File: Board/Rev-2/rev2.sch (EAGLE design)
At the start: 52 parts, among them IC1 74HC595N, T1 2N3904, T2 2N3904, T3 2N3904, T4 2N3904, T5 2N3904, T6 2N3904, T7 2N3904, T8 2N3904

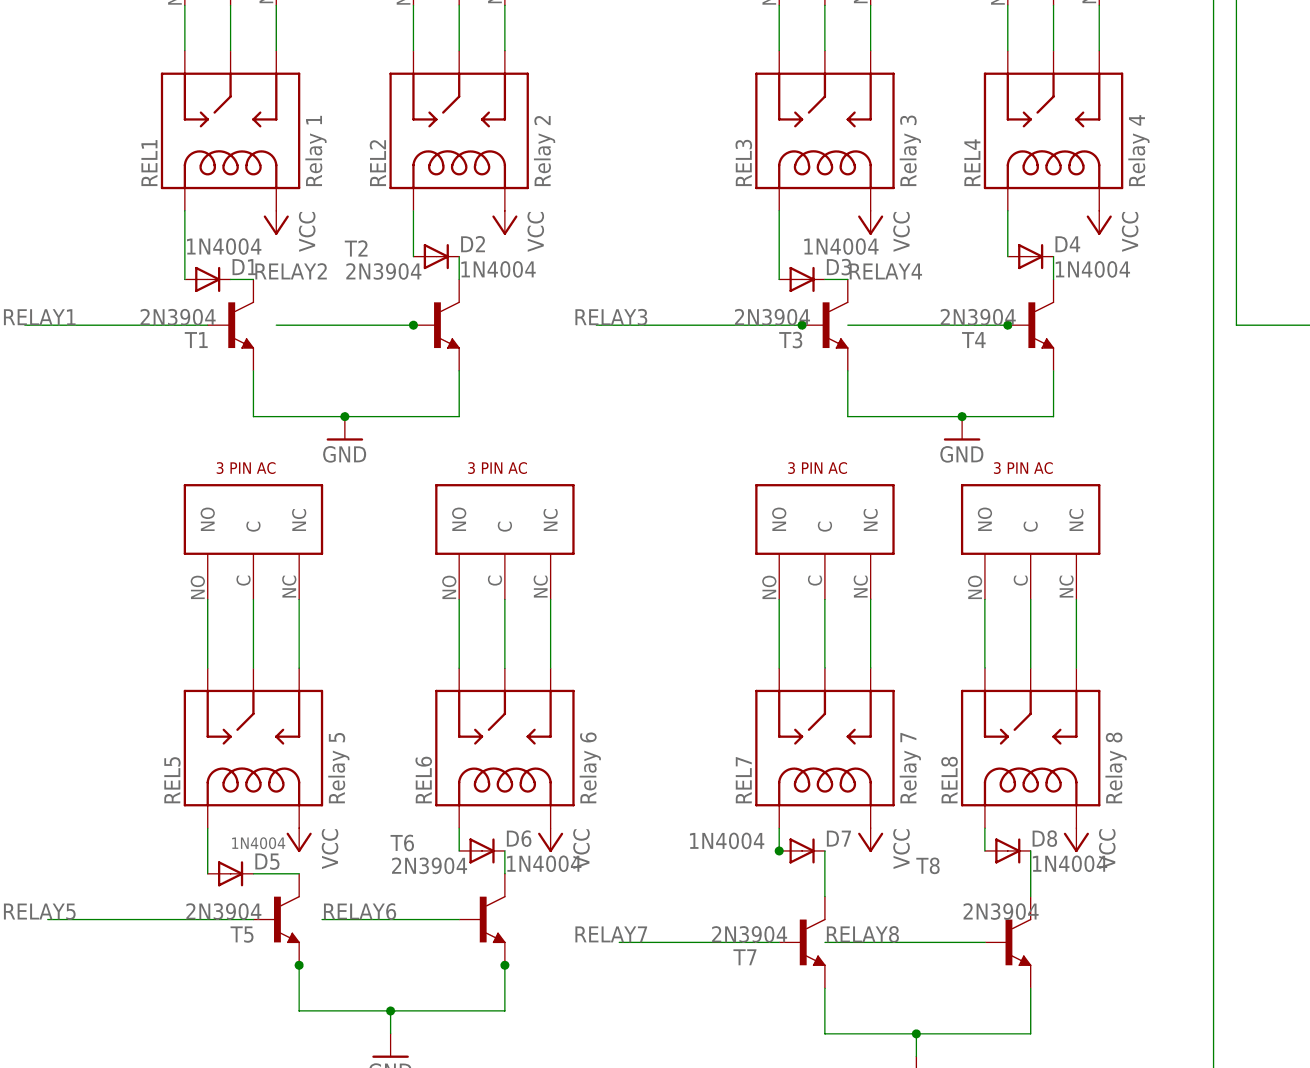
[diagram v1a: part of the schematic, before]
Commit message: Board Updates
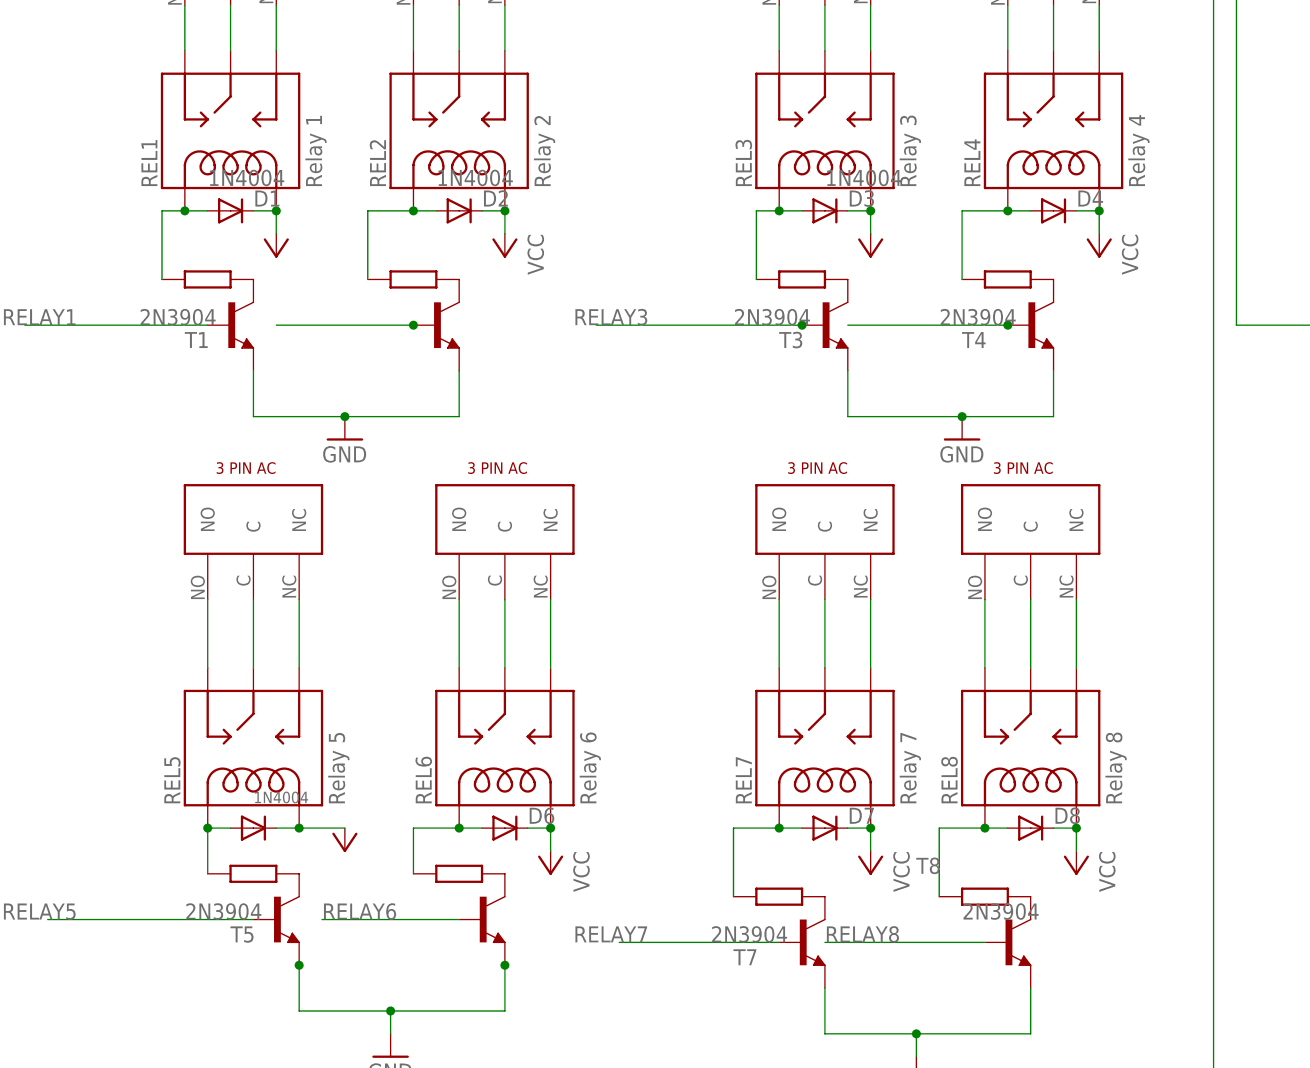
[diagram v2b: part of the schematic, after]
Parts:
- added LIMIT_REG_1, LIMIT_REG_2, LIMIT_REG_3, LIMIT_REG_4, LIMIT_REG_5, LIMIT_REG_6, LIMIT_REG_7, LIMIT_REG_8: 10 ohm, resistor:R-EU_0204/7
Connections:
- removed net N$47: D1.C, T1.C
- removed net N$48: D2.C, T2.C
- removed net N$49: D3.C, T3.C
- removed net N$50: D4.C, T4.C
- removed net N$51: D8.C, T8.C
- removed net N$52: D7.C, T7.C
- removed net N$53: D6.C, T6.C
- removed net N$54: D5.A, REL5.COIL1
- new net N$30: LIMIT_REG_1.1, T1.C
- new net N$32: LIMIT_REG_3.1, T3.C
- new net N$33: LIMIT_REG_2.1, T2.C
- new net N$34: LIMIT_REG_4.1, T4.C
- new net N$35: LIMIT_REG_8.1, T8.C
- new net N$36: LIMIT_REG_7.1, T7.C
- new net N$37: LIMIT_REG_6.1, T6.C
- new net N$38: LIMIT_REG_5.1, T5.C
- net N$1: now also D5.A, LIMIT_REG_5.2, REL5.COIL1; no longer D1.A, REL1.COIL1
- net N$2: now also D6.A, LIMIT_REG_6.2, REL6.COIL1; no longer D2.A, REL2.COIL1
- net N$3: now also D7.A, LIMIT_REG_7.2, REL7.COIL1; no longer D3.A, REL3.COIL1
- net N$4: now also D8.A, LIMIT_REG_8.2, REL8.COIL1; no longer D4.A, REL4.COIL1
- net N$5: now also D4.A, LIMIT_REG_4.2, REL4.COIL1; no longer D5.C, T5.C
- net N$6: now also D3.A, LIMIT_REG_3.2, REL3.COIL1; no longer D6.A, REL6.COIL1
- net N$8: now also D2.A, LIMIT_REG_2.2, REL2.COIL1; no longer D7.A, REL7.COIL1
- net N$9: now also D1.A, LIMIT_REG_1.2, REL1.COIL1; no longer D8.A, REL8.COIL1
- net VCC: now also D1.C, D2.C, D3.C, D4.C, D5.C, D6.C, D7.C, D8.C
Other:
- moved on the sheet: D1, D2, D3, D4, D6, D7, D8

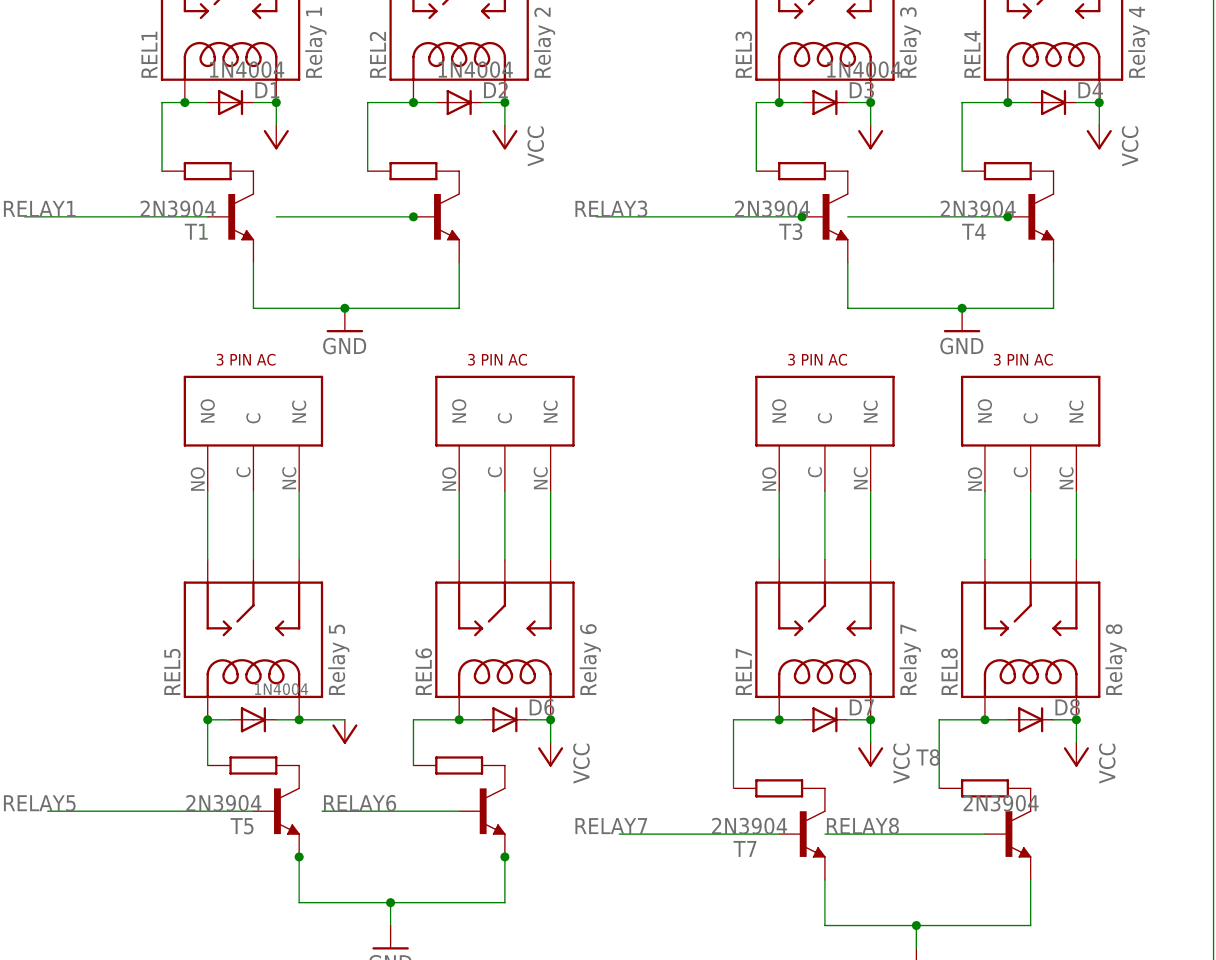
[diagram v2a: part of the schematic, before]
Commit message: Board Updates
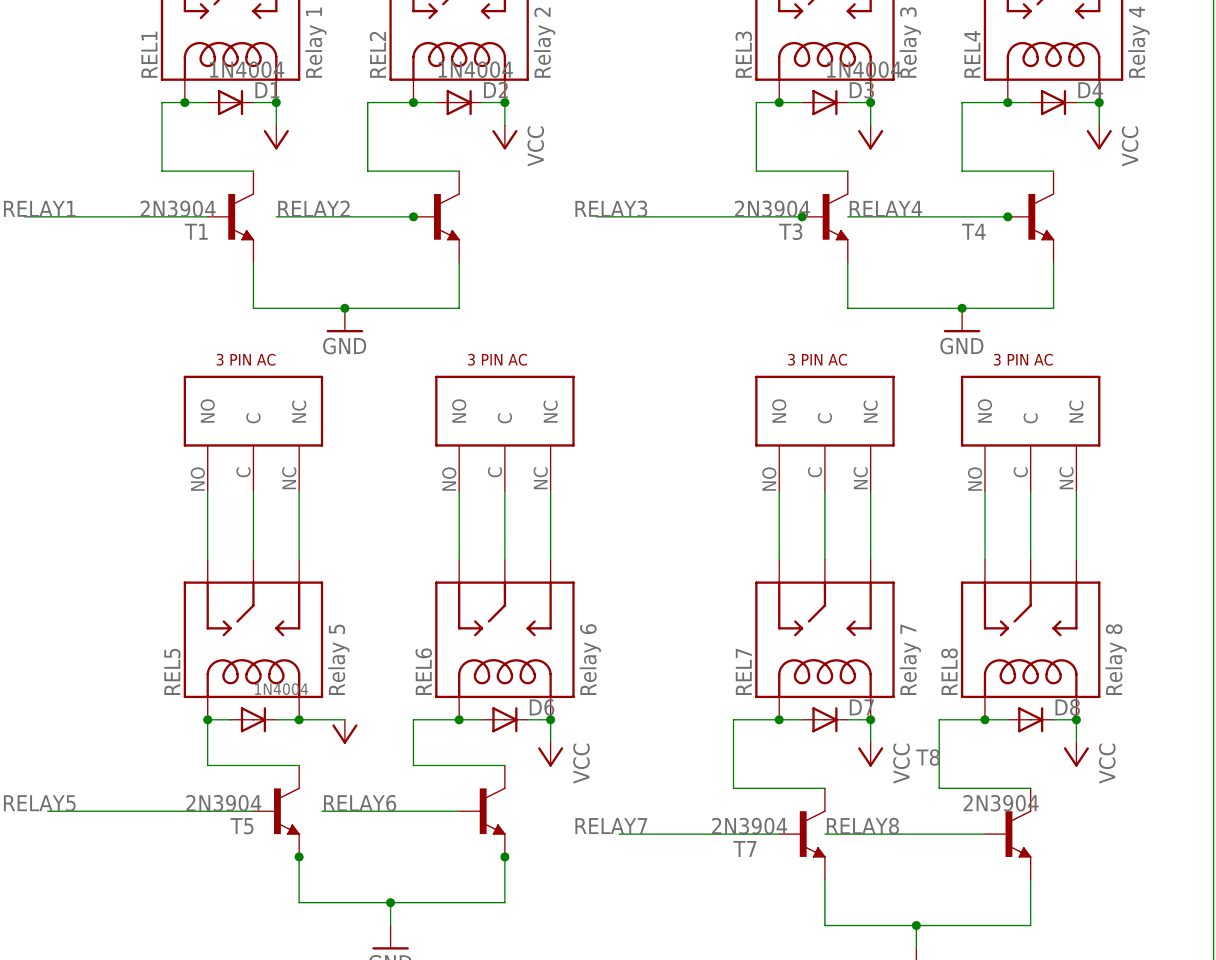
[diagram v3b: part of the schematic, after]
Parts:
- removed LIMIT_REG_1, LIMIT_REG_2, LIMIT_REG_3, LIMIT_REG_4, LIMIT_REG_5, LIMIT_REG_6, LIMIT_REG_7, LIMIT_REG_8: 10 ohm, resistor:R-EU_0204/7
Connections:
- removed net N$30: LIMIT_REG_1.1, T1.C
- removed net N$32: LIMIT_REG_3.1, T3.C
- removed net N$33: LIMIT_REG_2.1, T2.C
- removed net N$34: LIMIT_REG_4.1, T4.C
- removed net N$35: LIMIT_REG_8.1, T8.C
- removed net N$36: LIMIT_REG_7.1, T7.C
- removed net N$37: LIMIT_REG_6.1, T6.C
- removed net N$38: LIMIT_REG_5.1, T5.C
- net N$1: now also T5.C; no longer LIMIT_REG_5.2
- net N$2: now also T6.C; no longer LIMIT_REG_6.2
- net N$3: now also T7.C; no longer LIMIT_REG_7.2
- net N$4: now also T8.C; no longer LIMIT_REG_8.2
- net N$5: now also T4.C; no longer LIMIT_REG_4.2
- net N$6: now also T3.C; no longer LIMIT_REG_3.2
- net N$8: now also T2.C; no longer LIMIT_REG_2.2
- net N$9: now also T1.C; no longer LIMIT_REG_1.2
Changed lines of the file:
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@@
 <?xml version="1.0" encoding="utf-8"?>
 <!DOCTYPE eagle SYSTEM "eagle.dtd">
-<eagle version="9.6.2">
+<eagle version="9.3.0">
 <drawing>
 <settings>
@@
 </variantdefs>
 <classes>
-<class number="0" name="default" width="0" drill="0">
+<class number="0" name="default" width="0.2" drill="0">
 <clearance class="0" value="0.205"/>
 </class>
@@
 <part name="9V11" library="supply1" library_urn="urn:adsk.eagle:library:371" deviceset="VCC" device=""/>
 <part name="9V12" library="supply1" library_urn="urn:adsk.eagle:library:371" deviceset="VCC" device=""/>
-<part name="LIMIT_REG_1" library="resistor" library_urn="urn:adsk.eagle:library:348" deviceset="R-EU_" device="0204/7" package3d_urn="urn:adsk.eagle:package:25945/1" value="10 ohm"/>
-<part name="LIMIT_REG_3" library="resistor" library_urn="urn:adsk.eagle:library:348" deviceset="R-EU_" device="0204/7" package3d_urn="urn:adsk.eagle:package:25945/1" value="10 ohm"/>
-<part name="LIMIT_REG_2" library="resistor" library_urn="urn:adsk.eagle:library:348" deviceset="R-EU_" device="0204/7" package3d_urn="urn:adsk.eagle:package:25945/1" value="10 ohm"/>
-<part name="LIMIT_REG_4" library="resistor" library_urn="urn:adsk.eagle:library:348" deviceset="R-EU_" device="0204/7" package3d_urn="urn:adsk.eagle:package:25945/1" value="10 ohm"/>
-<part name="LIMIT_REG_8" library="resistor" library_urn="urn:adsk.eagle:library:348" deviceset="R-EU_" device="0204/7" package3d_urn="urn:adsk.eagle:package:25945/1" value="10 ohm"/>
-<part name="LIMIT_REG_7" library="resistor" library_urn="urn:adsk.eagle:library:348" deviceset="R-EU_" device="0204/7" package3d_urn="urn:adsk.eagle:package:25945/1" value="10 ohm"/>
-<part name="LIMIT_REG_6" library="resistor" library_urn="urn:adsk.eagle:library:348" deviceset="R-EU_" device="0204/7" package3d_urn="urn:adsk.eagle:package:25945/1" value="10 ohm"/>
-<part name="LIMIT_REG_5" library="resistor" library_urn="urn:adsk.eagle:library:348" deviceset="R-EU_" device="0204/7" package3d_urn="urn:adsk.eagle:package:25945/1" value="10 ohm"/>
 </parts>
 <sheets>
@@
 <instance part="T4" gate="G$1" x="281.94" y="76.2" smashed="yes">
 <attribute name="NAME" x="274.32" y="73.66" size="1.778" layer="95"/>
-<attribute name="VALUE" x="271.78" y="76.2" size="1.778" layer="96"/>
 </instance>
 <instance part="T6" gate="G$1" x="220.98" y="10.16" smashed="yes"/>
@@
 <attribute name="VALUE" x="86.36" y="91.44" size="1.778" layer="96"/>
 </instance>
-<instance part="LIMIT_REG_1" gate="G$1" x="190.5" y="81.28" smashed="yes" rot="R180"/>
-<instance part="LIMIT_REG_3" gate="G$1" x="256.54" y="81.28" smashed="yes" rot="R180"/>
-<instance part="LIMIT_REG_2" gate="G$1" x="213.36" y="81.28" smashed="yes" rot="R180"/>
-<instance part="LIMIT_REG_4" gate="G$1" x="279.4" y="81.28" smashed="yes" rot="R180"/>
-<instance part="LIMIT_REG_8" gate="G$1" x="276.86" y="12.7" smashed="yes" rot="R180"/>
-<instance part="LIMIT_REG_7" gate="G$1" x="254" y="12.7" smashed="yes" rot="R180"/>
-<instance part="LIMIT_REG_6" gate="G$1" x="218.44" y="15.24" smashed="yes" rot="R180"/>
-<instance part="LIMIT_REG_5" gate="G$1" x="195.58" y="15.24" smashed="yes" rot="R180"/>
 </instances>
 <busses>
@@
 <junction x="213.36" y="76.2"/>
 <wire x1="198.12" y1="76.2" x2="213.36" y2="76.2" width="0.1524" layer="91"/>
+<label x="198.12" y="76.2" size="1.778" layer="95"/>
 </segment>
 <segment>
@@
 <junction x="279.4" y="76.2"/>
 <wire x1="261.62" y1="76.2" x2="279.4" y2="76.2" width="0.1524" layer="91"/>
+<label x="261.62" y="76.2" size="1.778" layer="95"/>
 </segment>
 <segment>
@@
 <pinref part="D5" gate="1" pin="A"/>
 <wire x1="190.5" y1="20.32" x2="193.04" y2="20.32" width="0.1524" layer="91"/>
-<pinref part="LIMIT_REG_5" gate="G$1" pin="2"/>
 <wire x1="190.5" y1="15.24" x2="190.5" y2="20.32" width="0.1524" layer="91"/>
 <junction x="190.5" y="20.32"/>
+<pinref part="T5" gate="G$1" pin="C"/>
+<wire x1="190.5" y1="15.24" x2="200.66" y2="15.24" width="0.1524" layer="91"/>
 </segment>
 </net>
@@
 <pinref part="D6" gate="1" pin="A"/>
 <wire x1="218.44" y1="20.32" x2="220.98" y2="20.32" width="0.1524" layer="91"/>
-<pinref part="LIMIT_REG_6" gate="G$1" pin="2"/>
 <wire x1="213.36" y1="15.24" x2="213.36" y2="20.32" width="0.1524" layer="91"/>
 <wire x1="213.36" y1="20.32" x2="218.44" y2="20.32" width="0.1524" layer="91"/>
 <junction x="218.44" y="20.32"/>
+<pinref part="T6" gate="G$1" pin="C"/>
+<wire x1="213.36" y1="15.24" x2="223.52" y2="15.24" width="0.1524" layer="91"/>
 </segment>
 </net>
@@
 <pinref part="D7" gate="1" pin="A"/>
 <wire x1="254" y1="20.32" x2="256.54" y2="20.32" width="0.1524" layer="91"/>
-<pinref part="LIMIT_REG_7" gate="G$1" pin="2"/>
 <wire x1="248.92" y1="12.7" x2="248.92" y2="20.32" width="0.1524" layer="91"/>
 <wire x1="248.92" y1="20.32" x2="254" y2="20.32" width="0.1524" layer="91"/>
 <junction x="254" y="20.32"/>
+<pinref part="T7" gate="G$1" pin="C"/>
+<wire x1="248.92" y1="12.7" x2="259.08" y2="12.7" width="0.1524" layer="91"/>
 </segment>
 </net>
@@
 <pinref part="D8" gate="1" pin="A"/>
 <wire x1="276.86" y1="20.32" x2="279.4" y2="20.32" width="0.1524" layer="91"/>
-<pinref part="LIMIT_REG_8" gate="G$1" pin="2"/>
 <wire x1="271.78" y1="12.7" x2="271.78" y2="20.32" width="0.1524" layer="91"/>
 <wire x1="271.78" y1="20.32" x2="276.86" y2="20.32" width="0.1524" layer="91"/>
 <junction x="276.86" y="20.32"/>
+<pinref part="T8" gate="G$1" pin="C"/>
+<wire x1="271.78" y1="12.7" x2="281.94" y2="12.7" width="0.1524" layer="91"/>
 </segment>
 </net>
@@
 <pinref part="D4" gate="1" pin="A"/>
 <wire x1="279.4" y1="88.9" x2="281.94" y2="88.9" width="0.1524" layer="91"/>
-<pinref part="LIMIT_REG_4" gate="G$1" pin="2"/>
 <wire x1="274.32" y1="81.28" x2="274.32" y2="88.9" width="0.1524" layer="91"/>
 <wire x1="274.32" y1="88.9" x2="279.4" y2="88.9" width="0.1524" layer="91"/>
 <junction x="279.4" y="88.9"/>
+<pinref part="T4" gate="G$1" pin="C"/>
+<wire x1="274.32" y1="81.28" x2="284.48" y2="81.28" width="0.1524" layer="91"/>
 </segment>
 </net>
@@
 <pinref part="D3" gate="1" pin="A"/>
 <wire x1="254" y1="88.9" x2="256.54" y2="88.9" width="0.1524" layer="91"/>
-<pinref part="LIMIT_REG_3" gate="G$1" pin="2"/>
 <wire x1="251.46" y1="81.28" x2="251.46" y2="88.9" width="0.1524" layer="91"/>
 <wire x1="251.46" y1="88.9" x2="254" y2="88.9" width="0.1524" layer="91"/>
 <junction x="254" y="88.9"/>
+<pinref part="T3" gate="G$1" pin="C"/>
+<wire x1="251.46" y1="81.28" x2="261.62" y2="81.28" width="0.1524" layer="91"/>
 </segment>
 </net>
@@
 <pinref part="D2" gate="1" pin="A"/>
 <wire x1="213.36" y1="88.9" x2="215.9" y2="88.9" width="0.1524" layer="91"/>
-<pinref part="LIMIT_REG_2" gate="G$1" pin="2"/>
 <wire x1="208.28" y1="81.28" x2="208.28" y2="88.9" width="0.1524" layer="91"/>
 <wire x1="208.28" y1="88.9" x2="213.36" y2="88.9" width="0.1524" layer="91"/>
 <junction x="213.36" y="88.9"/>
+<pinref part="T2" gate="G$1" pin="C"/>
+<wire x1="208.28" y1="81.28" x2="218.44" y2="81.28" width="0.1524" layer="91"/>
 </segment>
 </net>
@@
 <pinref part="D1" gate="1" pin="A"/>
 <wire x1="187.96" y1="88.9" x2="190.5" y2="88.9" width="0.1524" layer="91"/>
-<pinref part="LIMIT_REG_1" gate="G$1" pin="2"/>
 <wire x1="185.42" y1="81.28" x2="185.42" y2="88.9" width="0.1524" layer="91"/>
 <wire x1="185.42" y1="88.9" x2="187.96" y2="88.9" width="0.1524" layer="91"/>
 <junction x="187.96" y="88.9"/>
-</segment>
-</net>
-<net name="N$30" class="0">
-<segment>
 <pinref part="T1" gate="G$1" pin="C"/>
-<pinref part="LIMIT_REG_1" gate="G$1" pin="1"/>
-</segment>
-</net>
-<net name="N$32" class="0">
-<segment>
-<pinref part="T3" gate="G$1" pin="C"/>
-<pinref part="LIMIT_REG_3" gate="G$1" pin="1"/>
-</segment>
-</net>
-<net name="N$33" class="0">
-<segment>
-<pinref part="T2" gate="G$1" pin="C"/>
-<pinref part="LIMIT_REG_2" gate="G$1" pin="1"/>
-</segment>
-</net>
-<net name="N$34" class="0">
-<segment>
-<pinref part="T4" gate="G$1" pin="C"/>
-<pinref part="LIMIT_REG_4" gate="G$1" pin="1"/>
-</segment>
-</net>
-<net name="N$35" class="0">
-<segment>
-<pinref part="T8" gate="G$1" pin="C"/>
-<pinref part="LIMIT_REG_8" gate="G$1" pin="1"/>
-</segment>
-</net>
-<net name="N$36" class="0">
-<segment>
-<pinref part="T7" gate="G$1" pin="C"/>
-<pinref part="LIMIT_REG_7" gate="G$1" pin="1"/>
-</segment>
-</net>
-<net name="N$37" class="0">
-<segment>
-<pinref part="T6" gate="G$1" pin="C"/>
-<pinref part="LIMIT_REG_6" gate="G$1" pin="1"/>
-</segment>
-</net>
-<net name="N$38" class="0">
-<segment>
-<pinref part="T5" gate="G$1" pin="C"/>
-<pinref part="LIMIT_REG_5" gate="G$1" pin="1"/>
-</segment>
-</net>
+<wire x1="185.42" y1="81.28" x2="195.58" y2="81.28" width="0.1524" layer="91"/>
+</segment>
+</net>
